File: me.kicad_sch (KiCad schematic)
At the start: 15 parts, among them M1 Motor_DC, Q1 AO3400A, SW1 SW_Push, SW2 SW_Push, SW3 SW_Push, SW4 SW_Push, SW5 SW_Push, SW6 SW_Push, U1 XIAO-RP2040-DIP

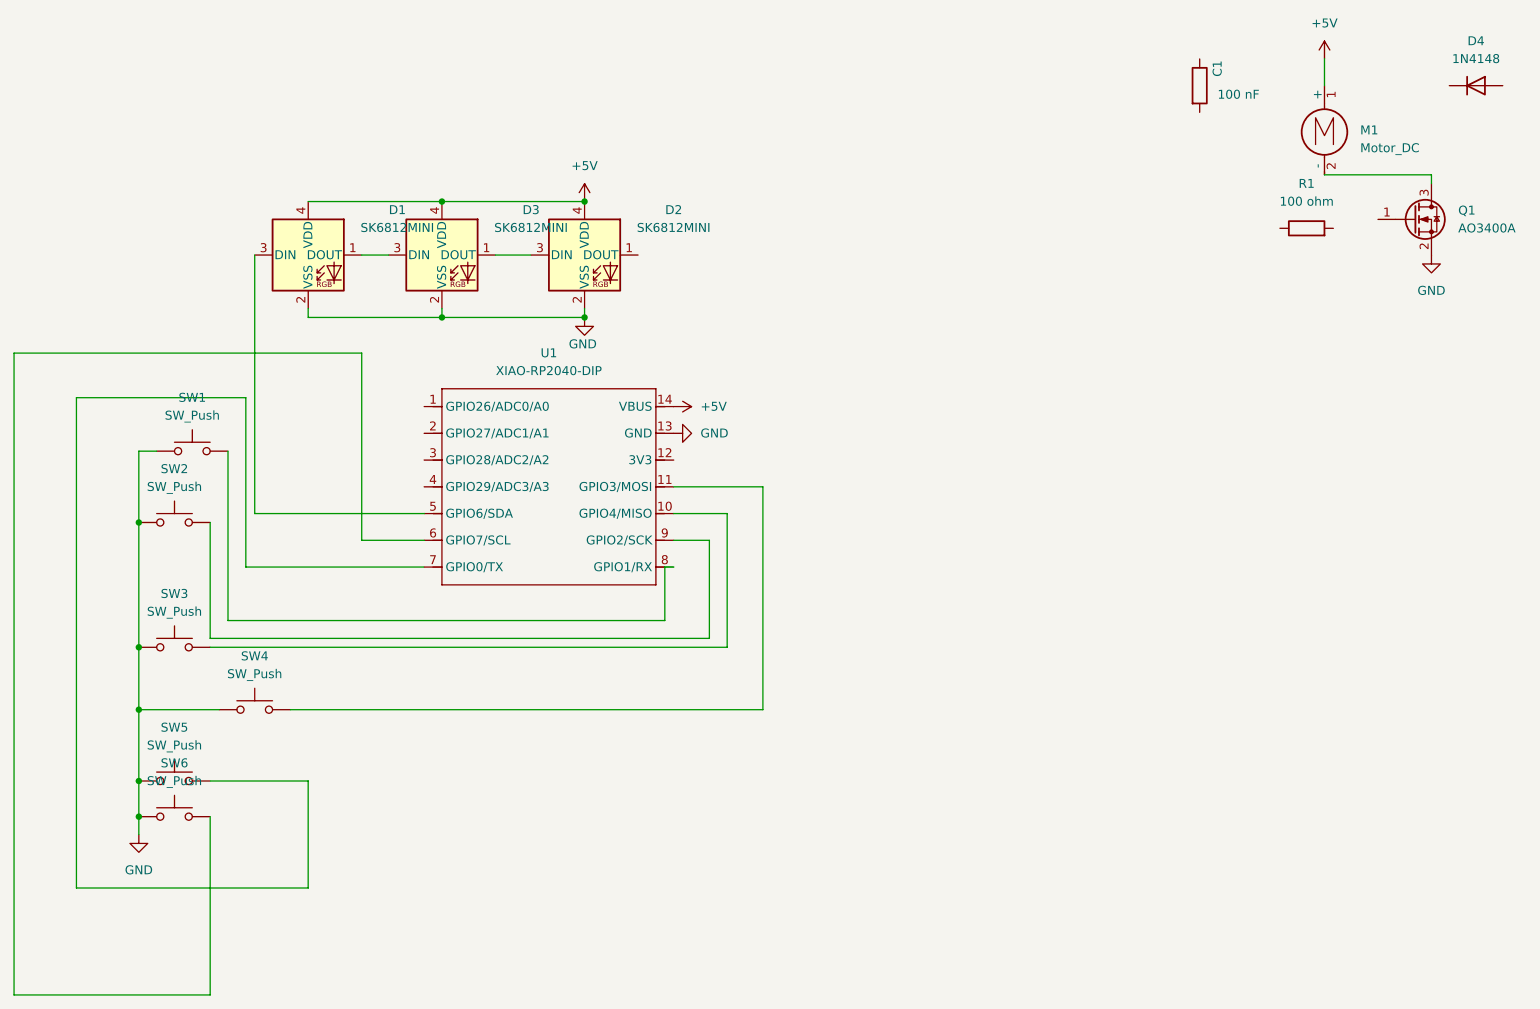
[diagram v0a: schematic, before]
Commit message: erwovnojerwnhvonwejvew
wrjgvwjngvloekr3w
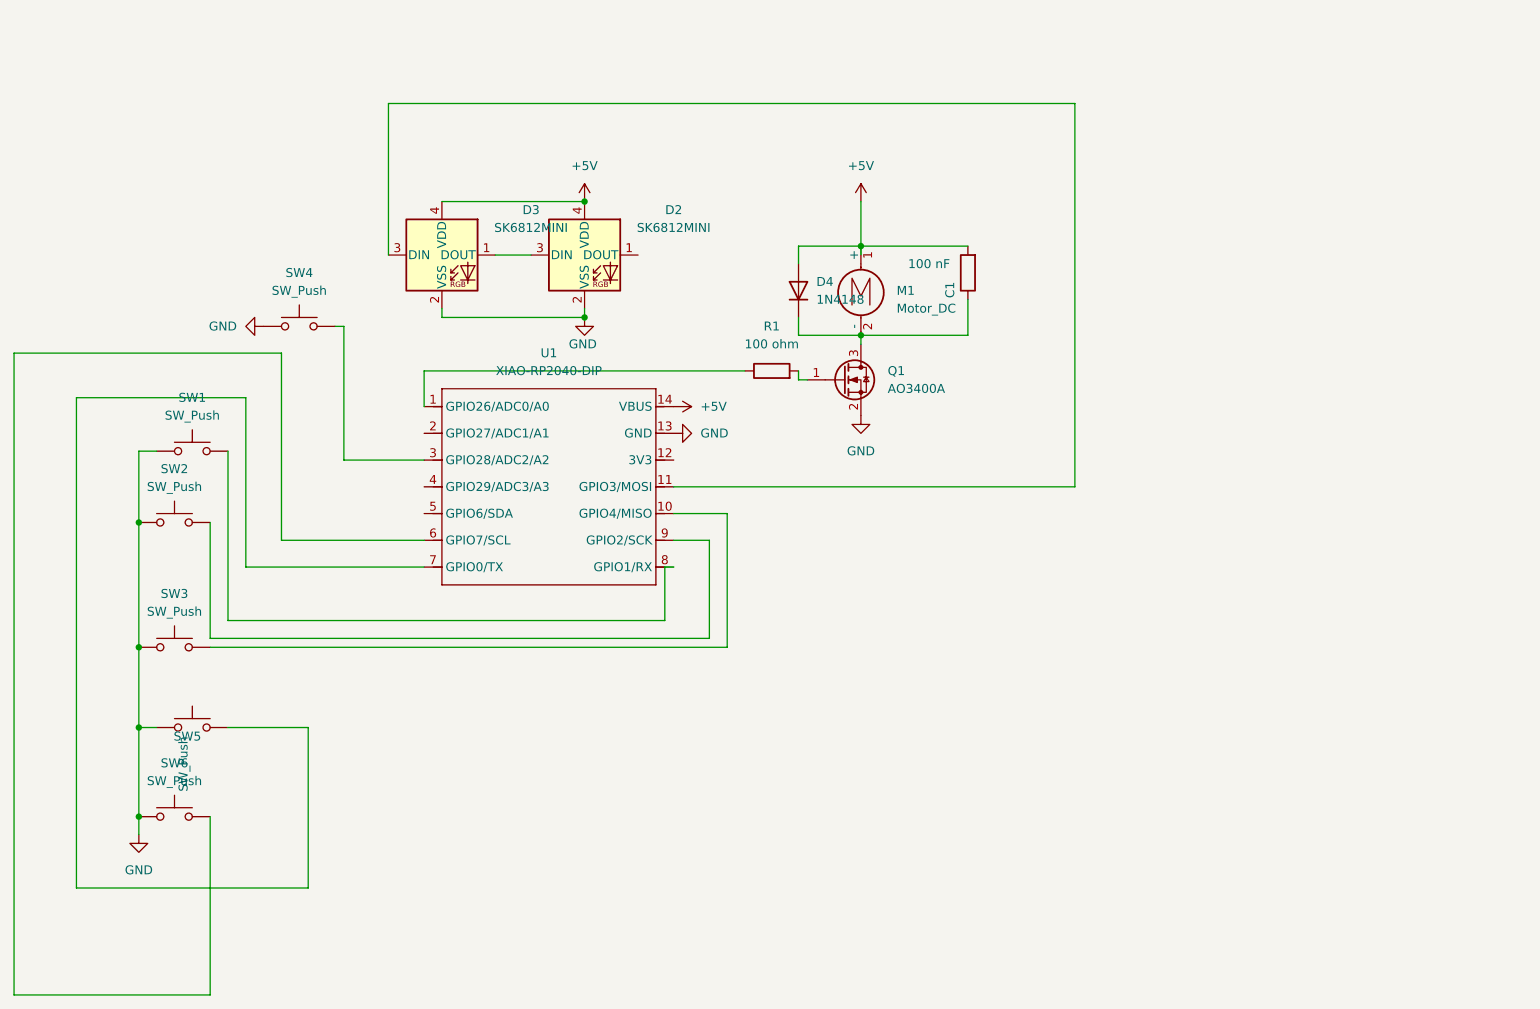
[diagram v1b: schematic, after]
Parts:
- removed D1: SK6812MINI, LED_SMD:LED_SK6812MINI_PLCC4_3.5x3.5mm_P1.75mm, symbol LED:SK6812MINI
- C1: footprint (none) -> Capacitor_SMD:C_0603_1608Metric
- M1: footprint (none) -> Connector_PinHeader_2.54mm:PinHeader_1x02_P2.54mm_Vertical
- R1: footprint (none) -> Resistor_SMD:R_0603_1608Metric
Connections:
- net +5V: now also C1.2, D4.2 (A)
- net at U1.1 (GPIO26/ADC0/A0): now also R1.1
- net at U1.11 (GPIO3/MOSI): now also D3.3 (DIN); no longer SW4.2
- net at U1.3 (GPIO28/ADC2/A2): now also SW4.2
- net at D4.1 (K): now also C1.1, M1.2 (-), Q1.3 (D)
- net at R1.2: now also Q1.1 (G)
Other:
- moved on the sheet: C1, D4, M1, Q1, R1, SW4, SW5
